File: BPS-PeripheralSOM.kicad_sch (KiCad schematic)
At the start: 30 parts, among them J2 Can_In, J5 Conn_02x10_Counter_Clockwise, J7 SWD, SW2 Reset, U1 STM32L431CBTx, Y1 8M

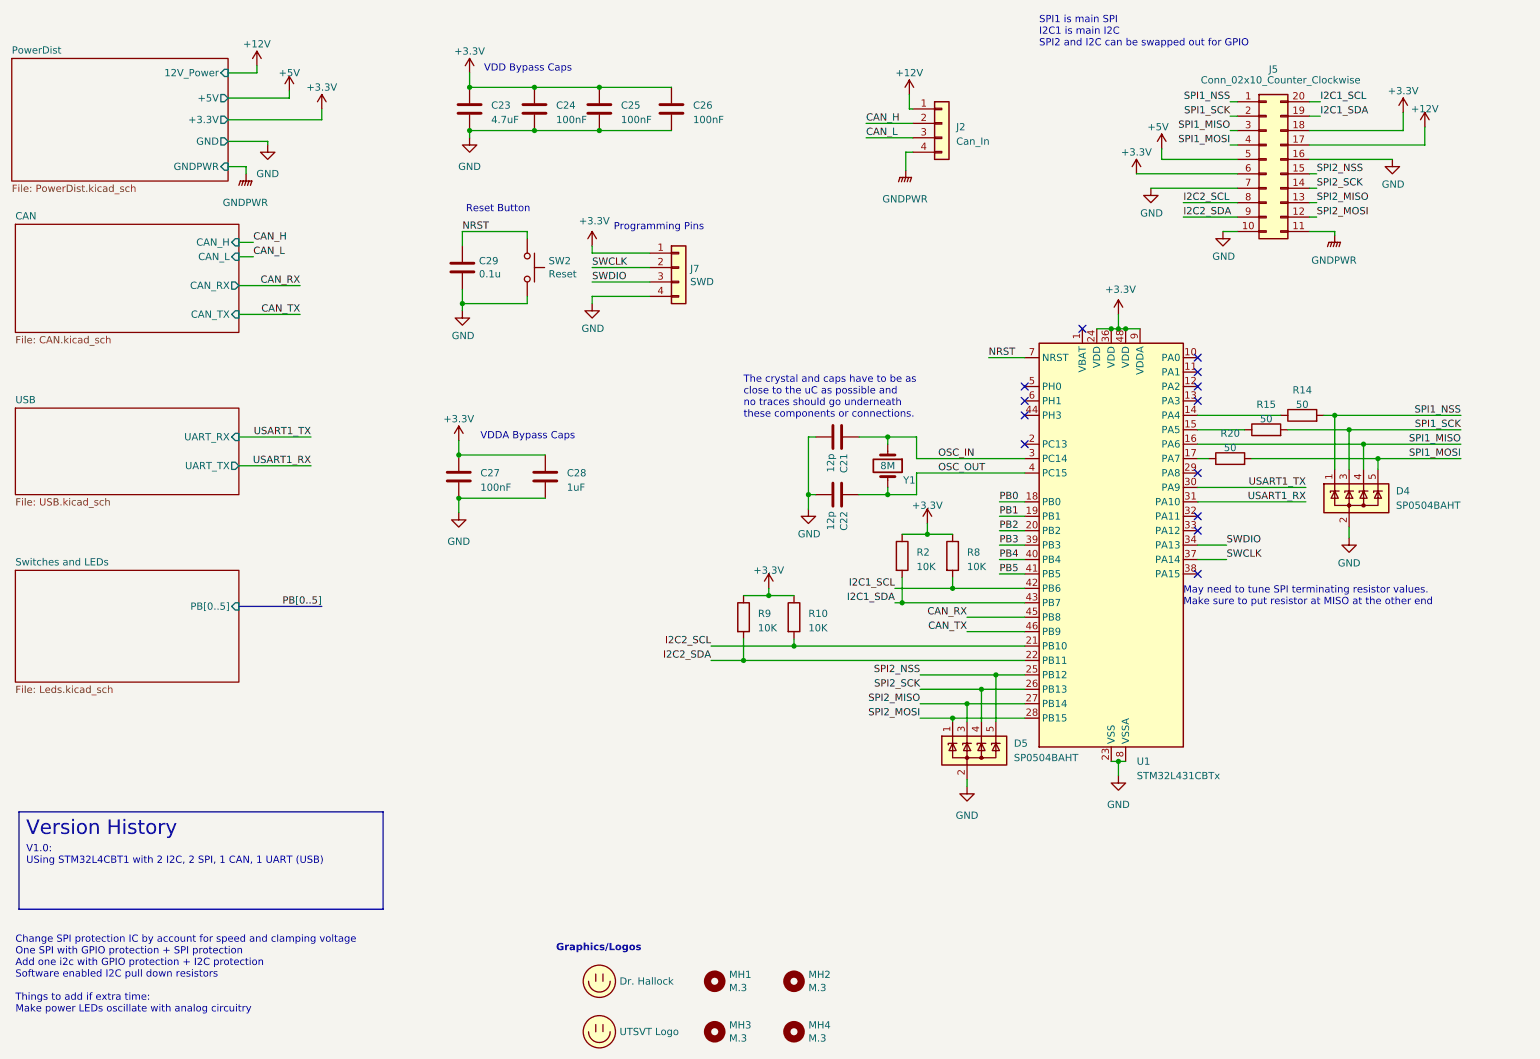
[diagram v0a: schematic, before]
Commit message: add 3.3v tvs diode
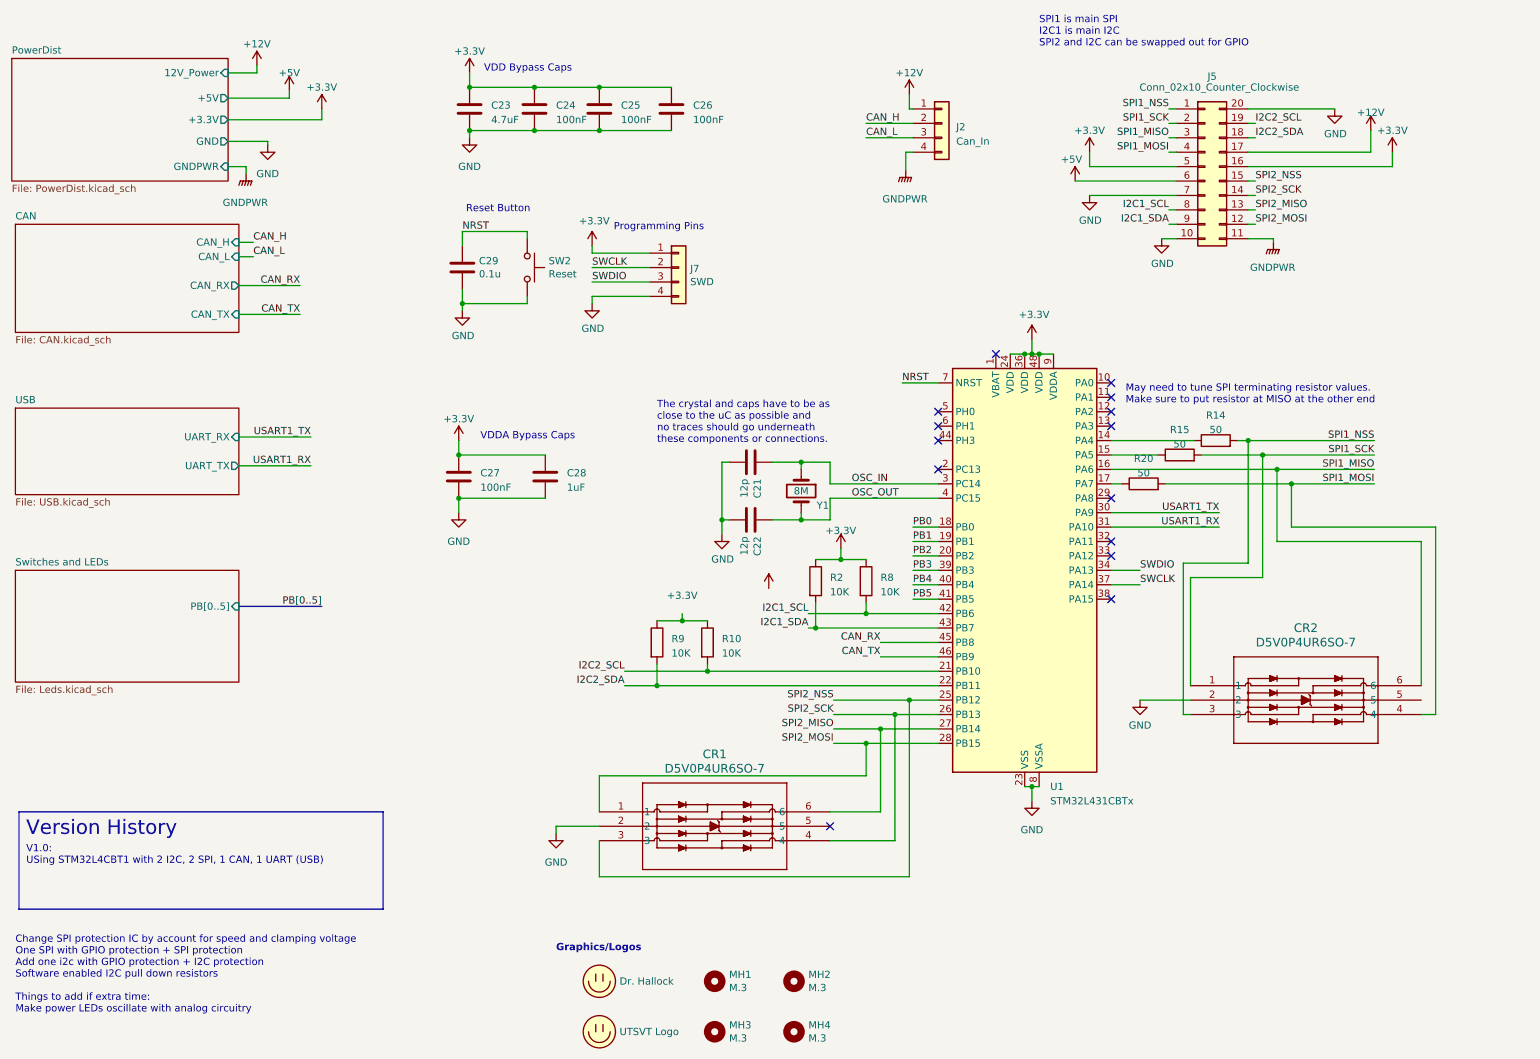
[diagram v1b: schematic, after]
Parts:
- removed D4, D5: SP0504BAHT, Package_TO_SOT_SMD:SOT-23-5, symbol Power_Protection:SP0504BAHT
- added CR1, CR2: D5V0P4UR6SO-7, UTSVT_ICs:SOT26_DIO, symbol utsvt-chips:D5V0P4UR6SO-7
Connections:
- net +3.3V: now also J5.16 (Pin_16), J5.5 (Pin_5); no longer J5.18 (Pin_18), J5.6 (Pin_6), R10.1, R9.1
- net +5V: now also J5.6 (Pin_6); no longer J5.5 (Pin_5)
- net GND: now also J5.20 (Pin_20), CR1.2, CR2.2; no longer J5.16 (Pin_16)
- net I2C1_SCL: now also J5.8 (Pin_8); no longer J5.20 (Pin_20)
- net I2C1_SDA: now also J5.9 (Pin_9); no longer J5.19 (Pin_19)
- net I2C2_SCL: now also J5.19 (Pin_19); no longer J5.8 (Pin_8)
- net I2C2_SDA: now also J5.18 (Pin_18); no longer J5.9 (Pin_9)
- net SPI1_MISO: now also CR2.6
- net SPI1_MOSI: now also CR2.4
- net SPI1_NSS: now also CR2.3
- net SPI1_SCK: now also CR2.1
- net SPI2_MISO: now also CR1.6
- net SPI2_MOSI: now also CR1.1
- net SPI2_NSS: now also CR1.3
- net SPI2_SCK: now also CR1.4
- new net: R10.1, R9.1
- no-connect marks 13 -> 14
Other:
- moved on the sheet: C21, C22, J5, R10, R14, R15, R2, R20, R8, R9, U1, Y1
